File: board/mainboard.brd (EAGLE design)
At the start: 26.1 x 65.4 mm, 10 parts, among them U1 DWM1000

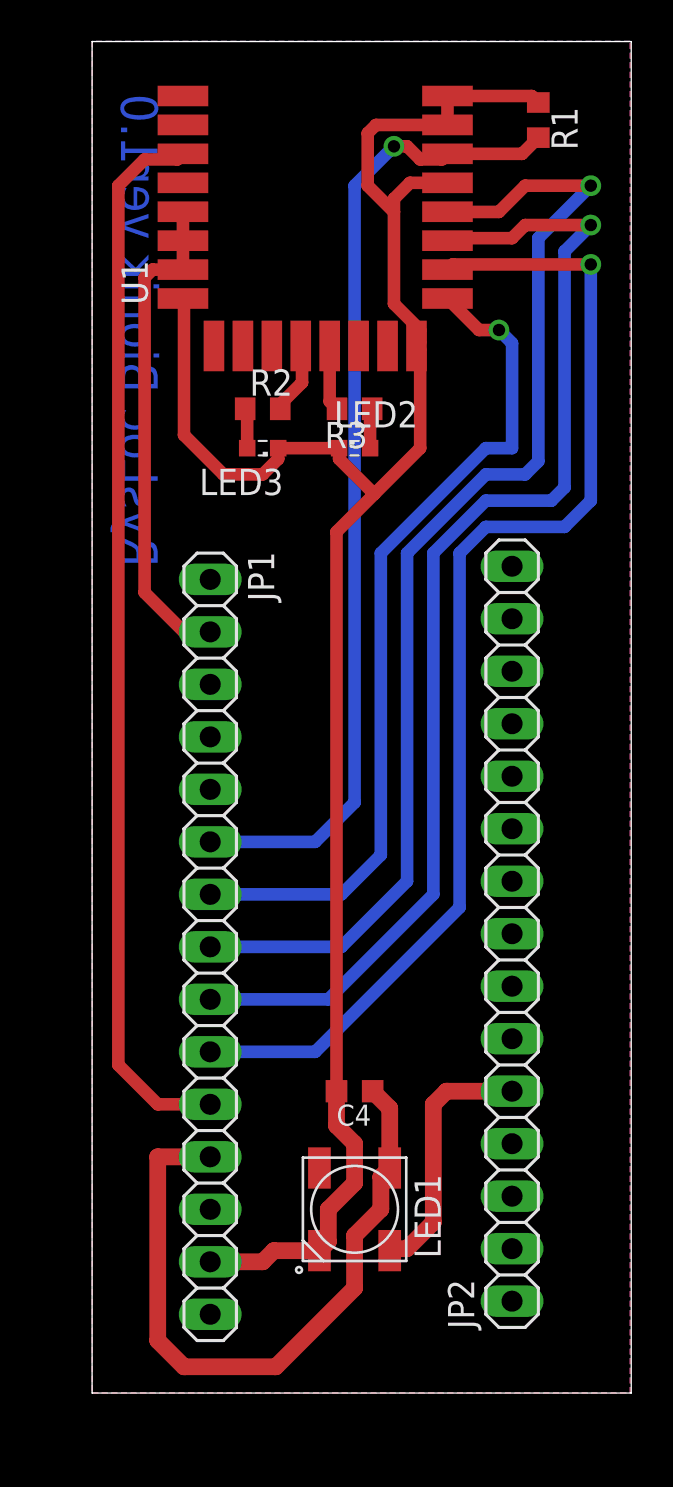
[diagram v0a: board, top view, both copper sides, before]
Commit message: powerplug and mountings
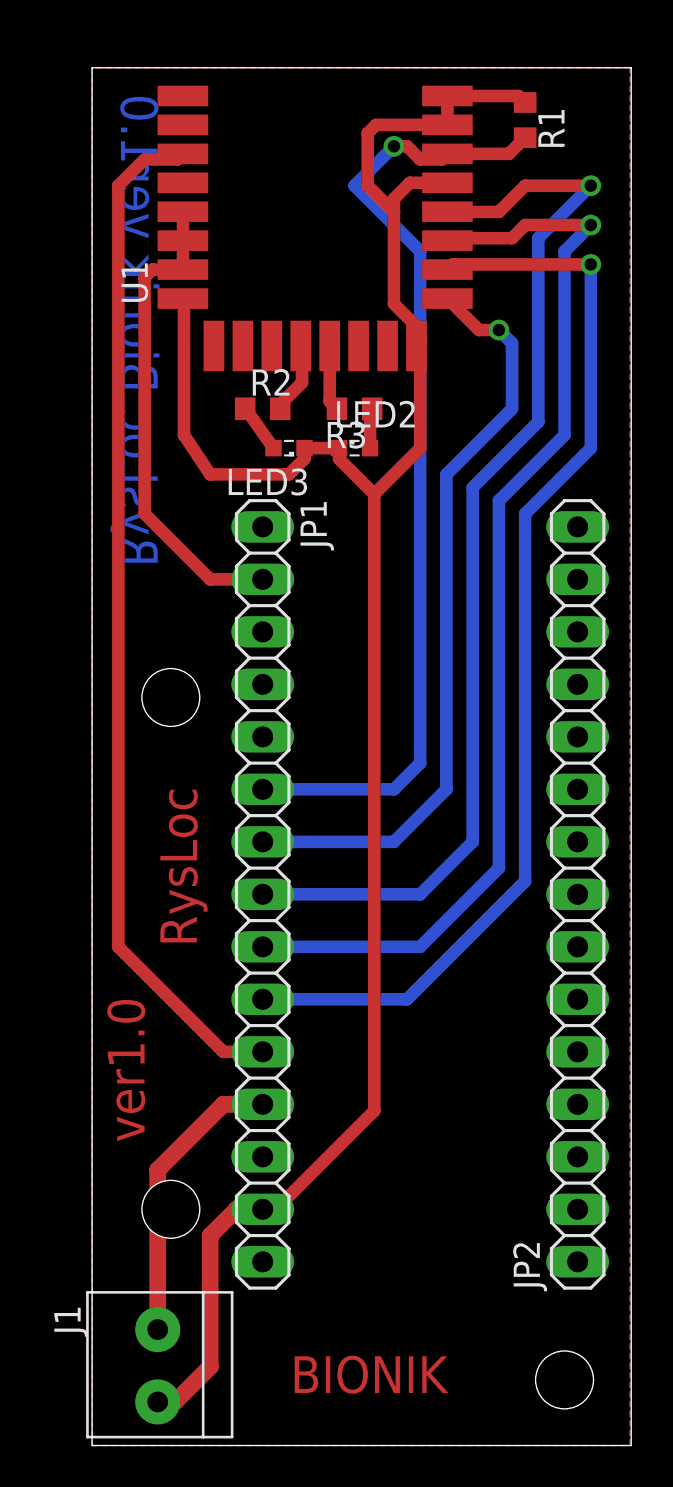
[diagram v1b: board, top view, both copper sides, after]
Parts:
- removed C4: 100n, rcl:C0603K
- removed LED1: WS2812B, WS2812B:WS2812B
- added J1: 1X2-3.5MM, adafruit:1X2-3.5MM
- moved JP2 3.70 mm to (91.4, 34.3)
- moved JP1 3.59 mm to (76.2, 34.3)
- moved LED3 1.27 mm to (77.5, 55.9)
- moved R1 0.63 mm to (88.9, 71.8)
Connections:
- net +5V: now also J1.1; no longer C4.1, LED1.VDD
- net GND: now also J1.2; no longer C4.2, LED1.VSS
- net LED1: no longer LED1.DIN
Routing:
- net +5V: track 33.6 -> 14.1 mm
- net LED1: track 12.5 -> 0.00 mm
- net GND: track 95.7 -> 101.2 mm
- net MOSI: track 58.0 -> 53.3 mm
- net MISO: track 57.5 -> 53.2 mm
- net CSN: track 41.2 -> 36.9 mm
- net SCK: track 56.8 -> 52.8 mm
- net DWMRES: track 51.5 -> 49.7 mm
- net IRQ: track 48.0 -> 47.1 mm
- net +3V3: track 24.0 -> 23.3 mm
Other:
- board size 26.1 x 65.4 mm -> 26.1 x 66.7 mm
- board text added: "BIONIK"
- board text added: "RysLoc"
- board text added: "ver1.0"
